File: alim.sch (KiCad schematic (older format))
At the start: 22 parts, among them IC10 74LS138, IC11 74LS138, IC12 74LS139, IC2 74LS09, IC5 74LS123, IC6 74LS393, IC7 74LS14, IC8 74LS04, IC9 74LS11

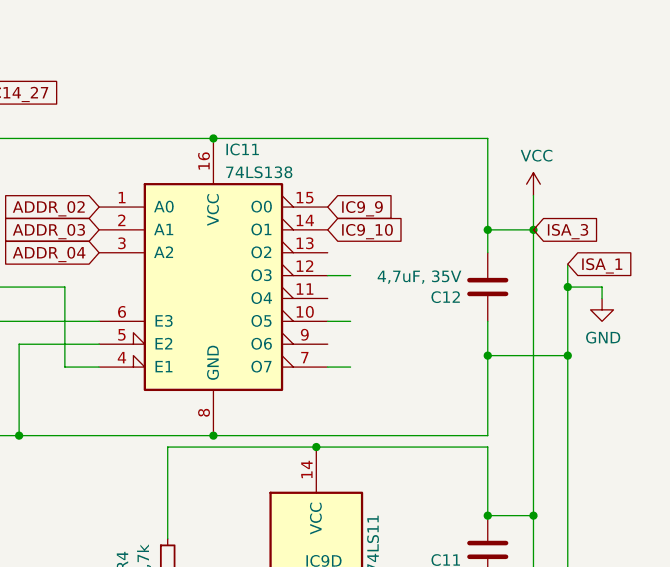
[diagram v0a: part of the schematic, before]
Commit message: les jumpers
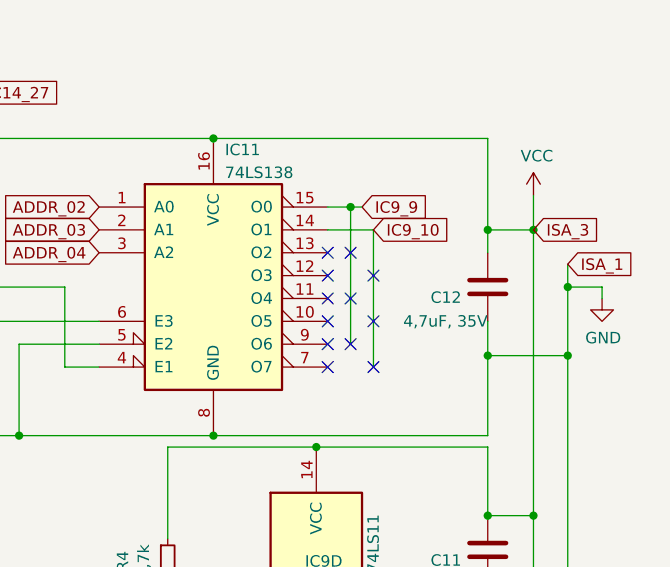
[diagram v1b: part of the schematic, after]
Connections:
- wire segments 122 -> 124
- no-connect marks 0 -> 12
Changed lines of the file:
@@
 AR Path="/61BDF4AD/6132D899" Ref="C12"  Part="1"
 F 0 "C12" H 6765 1896 50  0000 L CNN
-F 1 "4,7uF, 35V" H 6765 1805 50  0000 L CNN
+F 1 "4,7uF, 35V" H 6650 2000 50  0000 L CNN
 F 2 "Capacitor_THT:C_Disc_D4.3mm_W1.9mm_P5.00mm" H 6688 1700 50  0001 C CNN
 F 3 "~" H 6650 1850 50  0001 C CNN
@@
 Wire Wire Line
 	6650 1200 6650 1600
-Text GLabel 5950 1500 2    50   Input ~ 0
+Text GLabel 6100 1500 2    50   Input ~ 0
 IC9_9
 Connection ~ 5450 1200
@@
 Wire Wire Line
 	3550 1500 3800 1500
-Text GLabel 5950 1600 2    50   Input ~ 0
+Text GLabel 6150 1600 2    50   Input ~ 0
 IC9_10
 Wire Wire Line
@@
 Text GLabel 5500 4950 0    50   Input ~ 0
 DDD
-Wire Wire Line
-	5950 2000 6050 2000
-Wire Wire Line
-	5950 2200 6050 2200
-Wire Wire Line
-	5950 1800 6050 1800
+NoConn ~ 5950 2200
+NoConn ~ 5950 2000
+NoConn ~ 5950 1800
+NoConn ~ 6150 1800
+NoConn ~ 6150 2000
+NoConn ~ 6150 2200
+Wire Wire Line
+	6150 1600 6150 2200
+Wire Wire Line
+	5950 1600 6150 1600
+Wire Wire Line
+	6100 1500 6050 1500
+Wire Wire Line
+	6050 1500 6050 2100
+Connection ~ 6050 1500
+Wire Wire Line
+	6050 1500 5950 1500
+NoConn ~ 5950 1700
+NoConn ~ 6050 1700
+NoConn ~ 5950 1900
+NoConn ~ 6050 1900
+NoConn ~ 5950 2100
+NoConn ~ 6050 2100
 $EndSCHEMATC

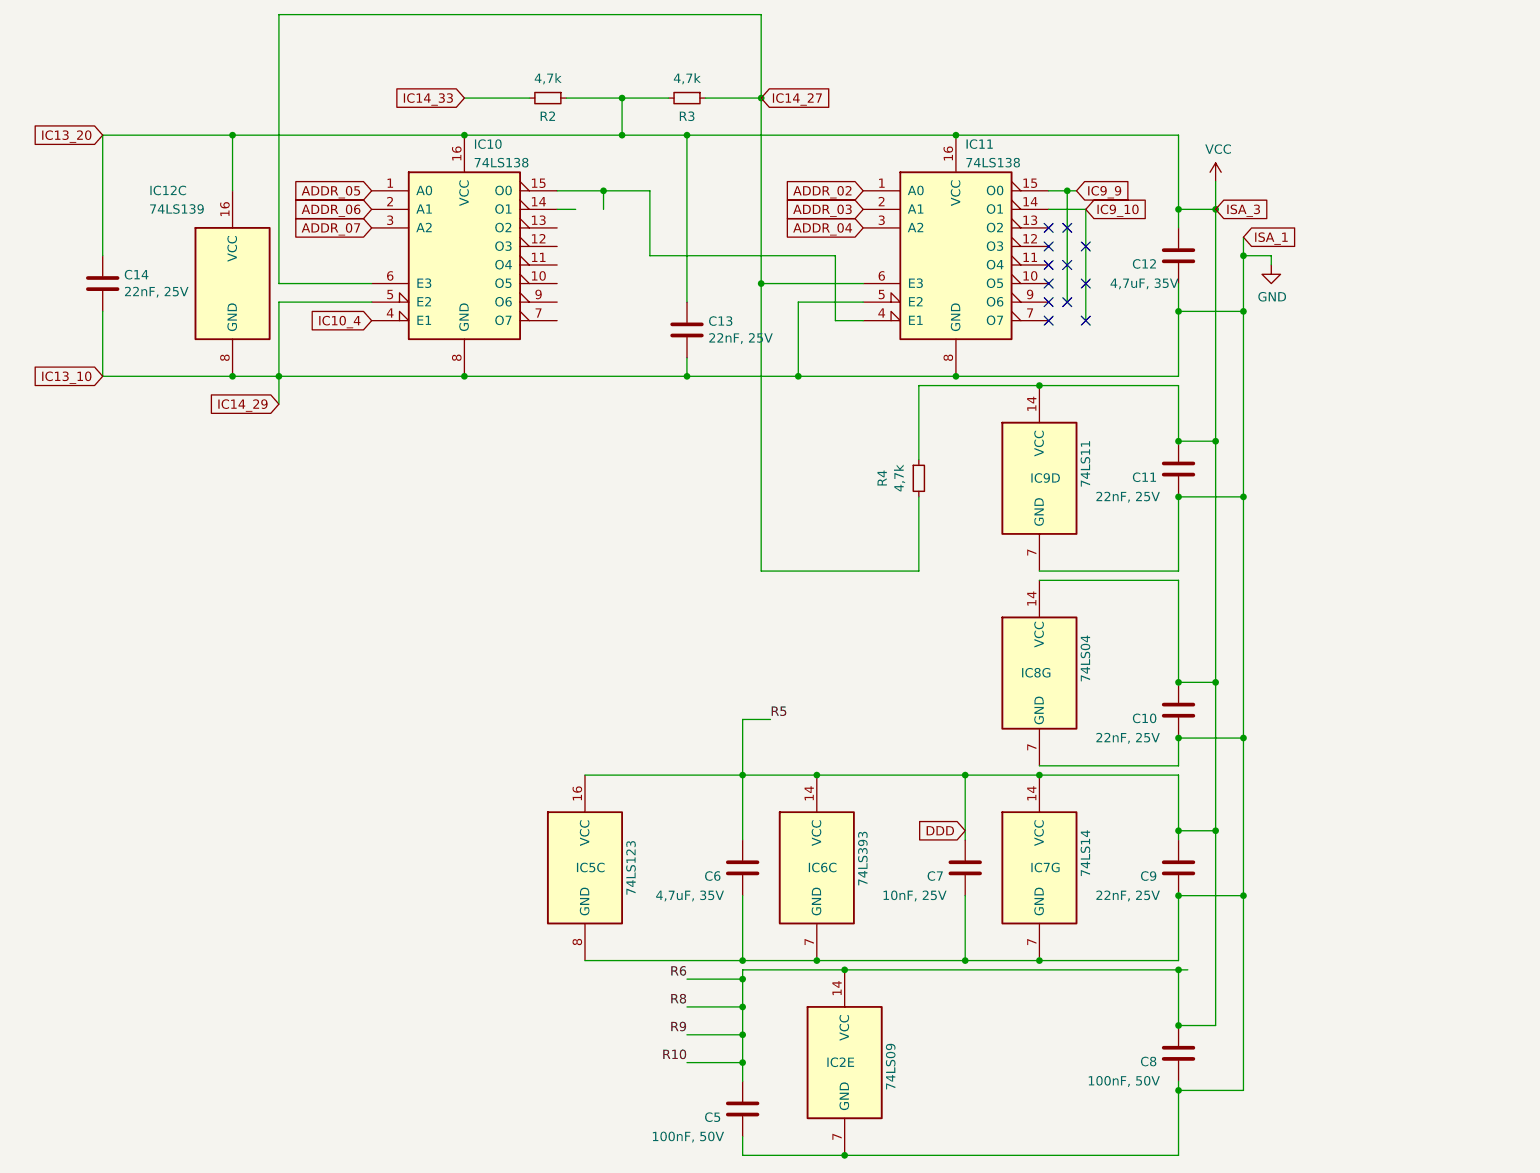
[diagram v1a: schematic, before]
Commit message: Schema de Freddy
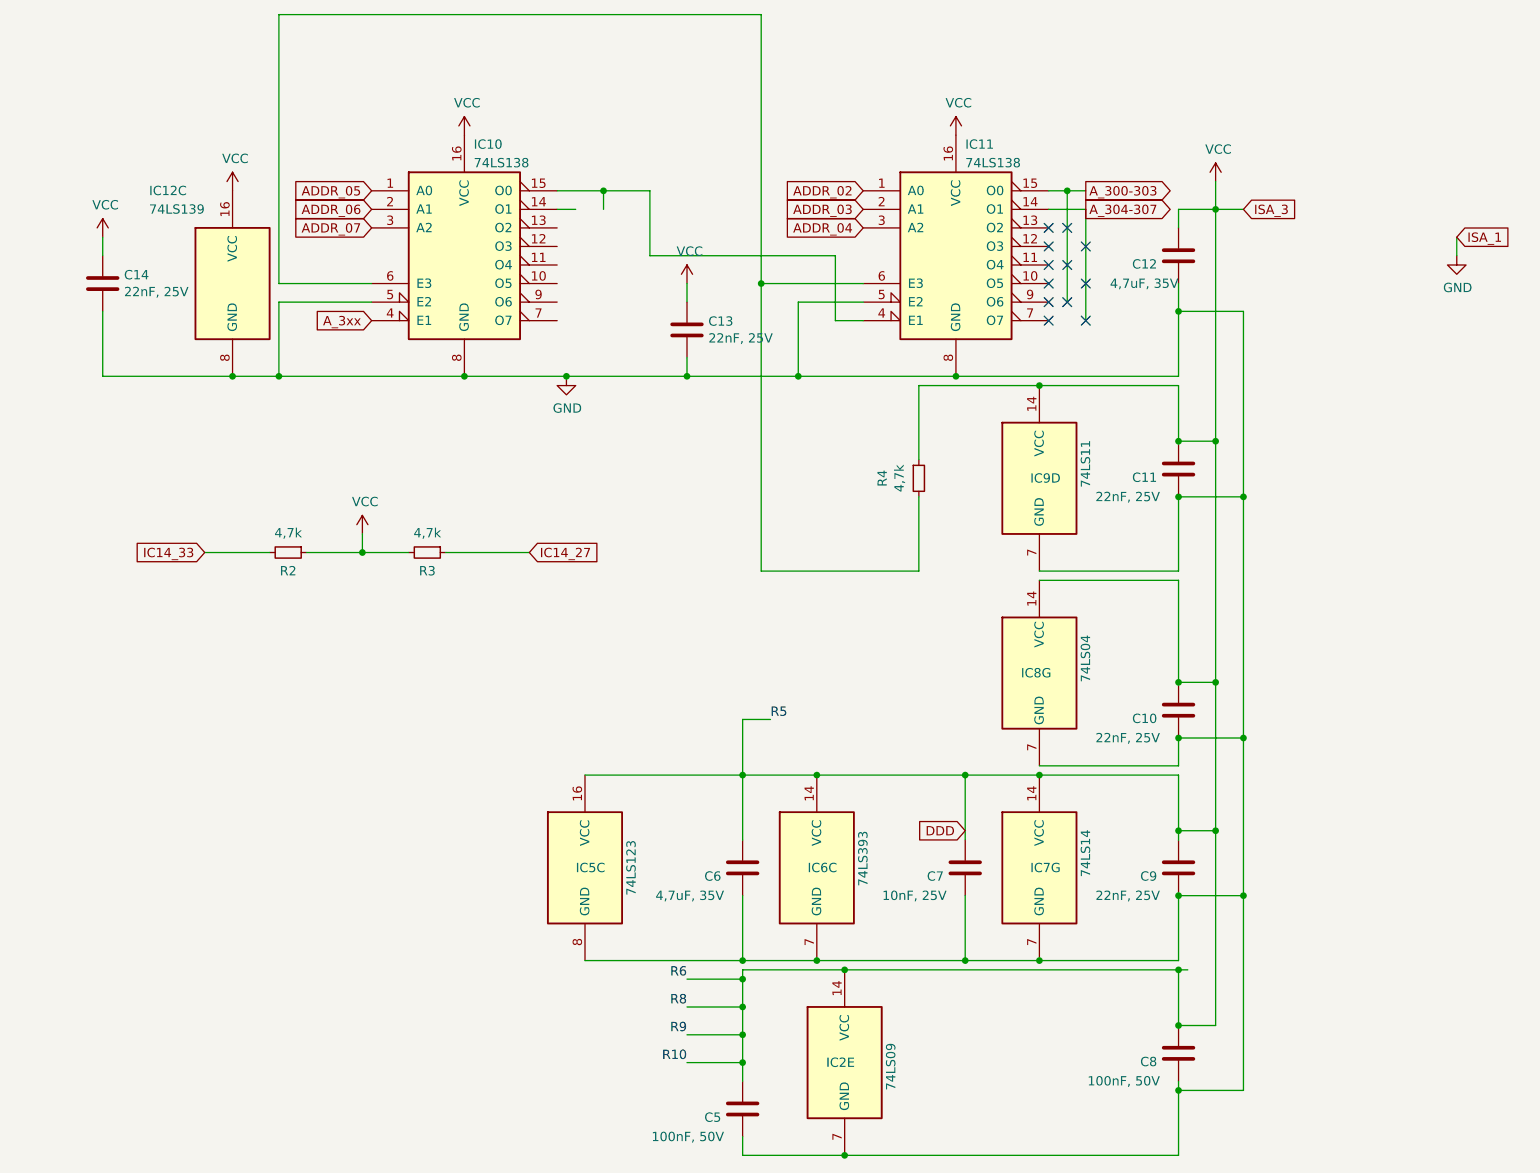
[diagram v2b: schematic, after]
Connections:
- net labels added: A_300-303, A_304-307, A_3xx
- net labels removed: IC10_4, IC13_10, IC13_20, IC14_29, IC9_10, IC9_9
- wire segments 124 -> 113
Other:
- moved on the sheet: R2, R3
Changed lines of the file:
@@
 $Descr A4 11693 8268
 encoding utf-8
-Sheet 3 3
+Sheet 1 1
 Title ""
 Date ""
@@
 L power:GND #PWR?
 U 1 1 612D8F44
-P 7150 1900
-F 0 "#PWR?" H 7150 1650 50  0001 C CNN
-F 1 "GND" H 7155 1727 50  0000 C CNN
-F 2 "" H 7150 1900 50  0001 C CNN
-F 3 "" H 7150 1900 50  0001 C CNN
-	1    7150 1900
+P 3350 2500
+F 0 "#PWR?" H 3350 2250 50  0001 C CNN
+F 1 "GND" H 3355 2327 50  0000 C CNN
+F 2 "" H 3350 2500 50  0001 C CNN
+F 3 "" H 3350 2500 50  0001 C CNN
+	1    3350 2500
 	1    0    0    -1
 $EndComp
@@
 	6650 2850 6850 2850
 Connection ~ 6650 2850
-Text GLabel 7000 1750 2    50   Input ~ 0
+Text GLabel 8150 1750 2    50   Input ~ 0
 ISA_1
-Text GLabel 6850 1600 2    50   Input ~ 0
+Text GLabel 7000 1600 2    50   Input ~ 0
 ISA_3
 $Comp
 L Device:R_Small R?
 U 1 1 6132D869
-P 4000 1000
+P 2600 3450
 AR Path="/6126F7E9/6132D869" Ref="R?"  Part="1"
 AR Path="/61BDF4AD/6132D869" Ref="R3"  Part="1"
-F 0 "R3" V 4100 1000 50  0000 C CNN
-F 1 "4,7k" V 3895 1000 50  0000 C CNN
-F 2 "Resistor_THT:R_Axial_DIN0309_L9.0mm_D3.2mm_P12.70mm_Horizontal" H 4000 1000 50  0001 C CNN
-F 3 "~" H 4000 1000 50  0001 C CNN
-	1    4000 1000
+F 0 "R3" V 2700 3450 50  0000 C CNN
+F 1 "4,7k" V 2495 3450 50  0000 C CNN
+F 2 "Resistor_THT:R_Axial_DIN0309_L9.0mm_D3.2mm_P12.70mm_Horizontal" H 2600 3450 50  0001 C CNN
+F 3 "~" H 2600 3450 50  0001 C CNN
+	1    2600 3450
 	0    1    1    0
 $EndComp
@@
 AR Path="/6126F7E9/6132D88D" Ref="IC?"  Part="1"
 AR Path="/61BDF4AD/6132D88D" Ref="IC11"  Part="1"
+AR Path="/6132D88D" Ref="IC11"  Part="1"
 F 0 "IC11" H 5500 2350 50  0000 L CNN
 F 1 "74LS138" H 5500 2250 50  0000 L CNN
@@
 $EndComp
 Wire Wire Line
-	1550 1500 1550 1200
-Wire Wire Line
 	1800 2000 2300 2000
 Wire Wire Line
@@
 	1800 2500 2800 2500
 Wire Wire Line
-	2800 1200 3650 1200
-Connection ~ 2800 1200
-Connection ~ 3650 1200
-Wire Wire Line
-	4000 1200 4000 2100
-Text GLabel 4400 1000 2    50   Input ~ 0
-IC14_27
+	4000 2000 4000 2100
 Wire Wire Line
 	4850 5700 6650 5700
@@
 Wire Wire Line
 	4850 6700 6650 6700
-Wire Wire Line
-	7150 1850 7000 1850
 Connection ~ 6850 4950
 Wire Wire Line
@@
 Wire Wire Line
 	6650 2000 6650 2150
-Wire Wire Line
-	7000 1850 7000 2150
 Connection ~ 7000 3150
 Connection ~ 6850 2850
 Wire Wire Line
 	6850 1450 6850 1600
-Wire Wire Line
-	6650 1200 6650 1600
-Text GLabel 6100 1500 2    50   Input ~ 0
-IC9_9
-Connection ~ 5450 1200
-Wire Wire Line
-	5450 1200 6650 1200
+Text GLabel 6150 1500 2    50   Output ~ 0
+A_300-303
 Connection ~ 5450 2500
 Wire Wire Line
 	5450 2500 6650 2500
-Wire Wire Line
-	3650 1200 4000 1200
 Wire Wire Line
 	4600 2100 4600 2500
@@
 	4600 2500 5450 2500
 Wire Wire Line
-	4400 2000 4400 1000
-Wire Wire Line
 	5900 2550 5250 2550
 Wire Wire Line
@@
 Wire Wire Line
 	4400 3550 5250 3550
-Connection ~ 4400 2000
-Wire Wire Line
-	4400 2000 4950 2000
 $Comp
 L Device:R_Small R?
 U 1 1 614CCF22
-P 3250 1000
+P 1850 3450
 AR Path="/6126F7E9/614CCF22" Ref="R?"  Part="1"
 AR Path="/61BDF4AD/614CCF22" Ref="R2"  Part="1"
-F 0 "R2" V 3350 1000 50  0000 C CNN
-F 1 "4,7k" V 3145 1000 50  0000 C CNN
-F 2 "Resistor_THT:R_Axial_DIN0309_L9.0mm_D3.2mm_P12.70mm_Horizontal" H 3250 1000 50  0001 C CNN
-F 3 "~" H 3250 1000 50  0001 C CNN
-	1    3250 1000
+F 0 "R2" V 1950 3450 50  0000 C CNN
+F 1 "4,7k" V 1745 3450 50  0000 C CNN
+F 2 "Resistor_THT:R_Axial_DIN0309_L9.0mm_D3.2mm_P12.70mm_Horizontal" H 1850 3450 50  0001 C CNN
+F 3 "~" H 1850 3450 50  0001 C CNN
+	1    1850 3450
 	0    1    1    0
 $EndComp
 Wire Wire Line
 	7000 2150 6650 2150
-Connection ~ 7000 2150
 Wire Wire Line
 	7000 2150 7000 3150
@@
 Wire Wire Line
 	6650 1600 6850 1600
-Connection ~ 6650 1600
 Wire Wire Line
 	6650 1600 6650 1700
@@
 	6850 1600 6850 2850
 Wire Wire Line
-	4100 1000 4400 1000
-Wire Wire Line
-	3900 1000 3650 1000
-Wire Wire Line
-	3650 1000 3650 1200
-Wire Wire Line
-	3650 1000 3350 1000
-Connection ~ 3650 1000
-Text GLabel 2800 1000 0    50   Input ~ 0
+	2500 3450 2250 3450
+Wire Wire Line
+	2250 3450 1950 3450
+Connection ~ 2250 3450
+Text GLabel 1400 3450 0    50   Input ~ 0
 IC14_33
 Wire Wire Line
-	3150 1000 2800 1000
-Wire Wire Line
-	850  1200 850  1850
+	1750 3450 1400 3450
+Wire Wire Line
+	850  1750 850  1850
 Text GLabel 2300 2200 0    50   Input ~ 0
-IC10_4
-Connection ~ 4000 1200
-Wire Wire Line
-	4000 1200 5450 1200
+A_3xx
 Connection ~ 4000 2500
 Wire Wire Line
 	4000 2500 4600 2500
 Wire Wire Line
-	2800 2500 4000 2500
+	2800 2500 3350 2500
 Wire Wire Line
 	3550 1500 3550 1600
@@
 Wire Wire Line
 	3550 1500 3800 1500
-Text GLabel 6150 1600 2    50   Input ~ 0
-IC9_10
+Text GLabel 6150 1600 2    50   Output ~ 0
+A_304-307
 Wire Wire Line
 	7000 6350 6650 6350
@@
 Wire Wire Line
 	850  2500 1550 2500
-Connection ~ 1550 1200
-Wire Wire Line
-	1550 1200 2800 1200
-Wire Wire Line
-	850  1200 1550 1200
-Wire Wire Line
-	1800 2500 1800 2650
-Text GLabel 1800 2650 0    50   Input ~ 0
-IC14_29
-Text GLabel 850  2500 0    50   Input ~ 0
-IC13_10
-Text GLabel 850  1200 0    50   Input ~ 0
-IC13_20
 Wire Wire Line
 	1800 550  4400 550
 Wire Wire Line
-	4400 550  4400 1000
-Wire Wire Line
 	1800 550  1800 2000
-Connection ~ 4400 1000
-Wire Wire Line
-	7000 1750 7000 1850
-Connection ~ 7000 1850
-Wire Wire Line
-	7150 1850 7150 1900
+Wire Wire Line
+	8150 1750 8150 1850
 Text GLabel 5500 4950 0    50   Input ~ 0
 DDD
@@
 	5950 1600 6150 1600
 Wire Wire Line
-	6100 1500 6050 1500
+	6150 1500 6050 1500
 Wire Wire Line
 	6050 1500 6050 2100
@@
 NoConn ~ 5950 2100
 NoConn ~ 6050 2100
+Connection ~ 3350 2500
+Wire Wire Line
+	3350 2500 4000 2500
+$Comp
+L power:GND #PWR?
+U 1 1 61332220
+P 8150 1850
+F 0 "#PWR?" H 8150 1600 50  0001 C CNN
+F 1 "GND" H 8155 1677 50  0000 C CNN
+F 2 "" H 8150 1850 50  0001 C CNN
+F 3 "" H 8150 1850 50  0001 C CNN
+	1    8150 1850
+	1    0    0    -1
+$EndComp
+Wire Wire Line
+	7000 1600 6850 1600
+$Comp
+L power:VCC #PWR?
+U 1 1 6134655A
+P 5450 1200
+F 0 "#PWR?" H 5450 1050 50  0001 C CNN
+F 1 "VCC" H 5465 1373 50  0000 C CNN
+F 2 "" H 5450 1200 50  0001 C CNN
+F 3 "" H 5450 1200 50  0001 C CNN
+	1    5450 1200
+	1    0    0    -1
+$EndComp
+$Comp
+L power:VCC #PWR?
+U 1 1 6134C22C
+P 2250 3350
+F 0 "#PWR?" H 2250 3200 50  0001 C CNN
+F 1 "VCC" H 2265 3523 50  0000 C CNN
+F 2 "" H 2250 3350 50  0001 C CNN
+F 3 "" H 2250 3350 50  0001 C CNN
+	1    2250 3350
+	1    0    0    -1
+$EndComp
+Wire Wire Line
+	2250 3350 2250 3450
+$Comp
+L power:VCC #PWR?
+U 1 1 61355045
+P 4000 2000
+F 0 "#PWR?" H 4000 1850 50  0001 C CNN
+F 1 "VCC" H 4015 2173 50  0000 C CNN
+F 2 "" H 4000 2000 50  0001 C CNN
+F 3 "" H 4000 2000 50  0001 C CNN
+	1    4000 2000
+	1    0    0    -1
+$EndComp
+$Comp
+L power:VCC #PWR?
+U 1 1 61356035
+P 2800 1200
+F 0 "#PWR?" H 2800 1050 50  0001 C CNN
+F 1 "VCC" H 2815 1373 50  0000 C CNN
+F 2 "" H 2800 1200 50  0001 C CNN
+F 3 "" H 2800 1200 50  0001 C CNN
+	1    2800 1200
+	1    0    0    -1
+$EndComp
+Text GLabel 3150 3450 2    50   Input ~ 0
+IC14_27
+Wire Wire Line
+	3150 3450 2700 3450
+Wire Wire Line
+	4400 550  4400 2000
+Connection ~ 4400 2000
+Wire Wire Line
+	4400 2000 4950 2000
+$Comp
+L power:VCC #PWR?
+U 1 1 6137A5D8
+P 1550 1500
+F 0 "#PWR?" H 1550 1350 50  0001 C CNN
+F 1 "VCC" H 1565 1673 50  0000 C CNN
+F 2 "" H 1550 1500 50  0001 C CNN
+F 3 "" H 1550 1500 50  0001 C CNN
+	1    1550 1500
+	1    0    0    -1
+$EndComp
+$Comp
+L power:VCC #PWR?
+U 1 1 6137B0FA
+P 850 1750
+F 0 "#PWR?" H 850 1600 50  0001 C CNN
+F 1 "VCC" H 865 1923 50  0000 C CNN
+F 2 "" H 850 1750 50  0001 C CNN
+F 3 "" H 850 1750 50  0001 C CNN
+	1    850  1750
+	1    0    0    -1
+$EndComp
 $EndSCHEMATC

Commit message: Dernière version de Freddy
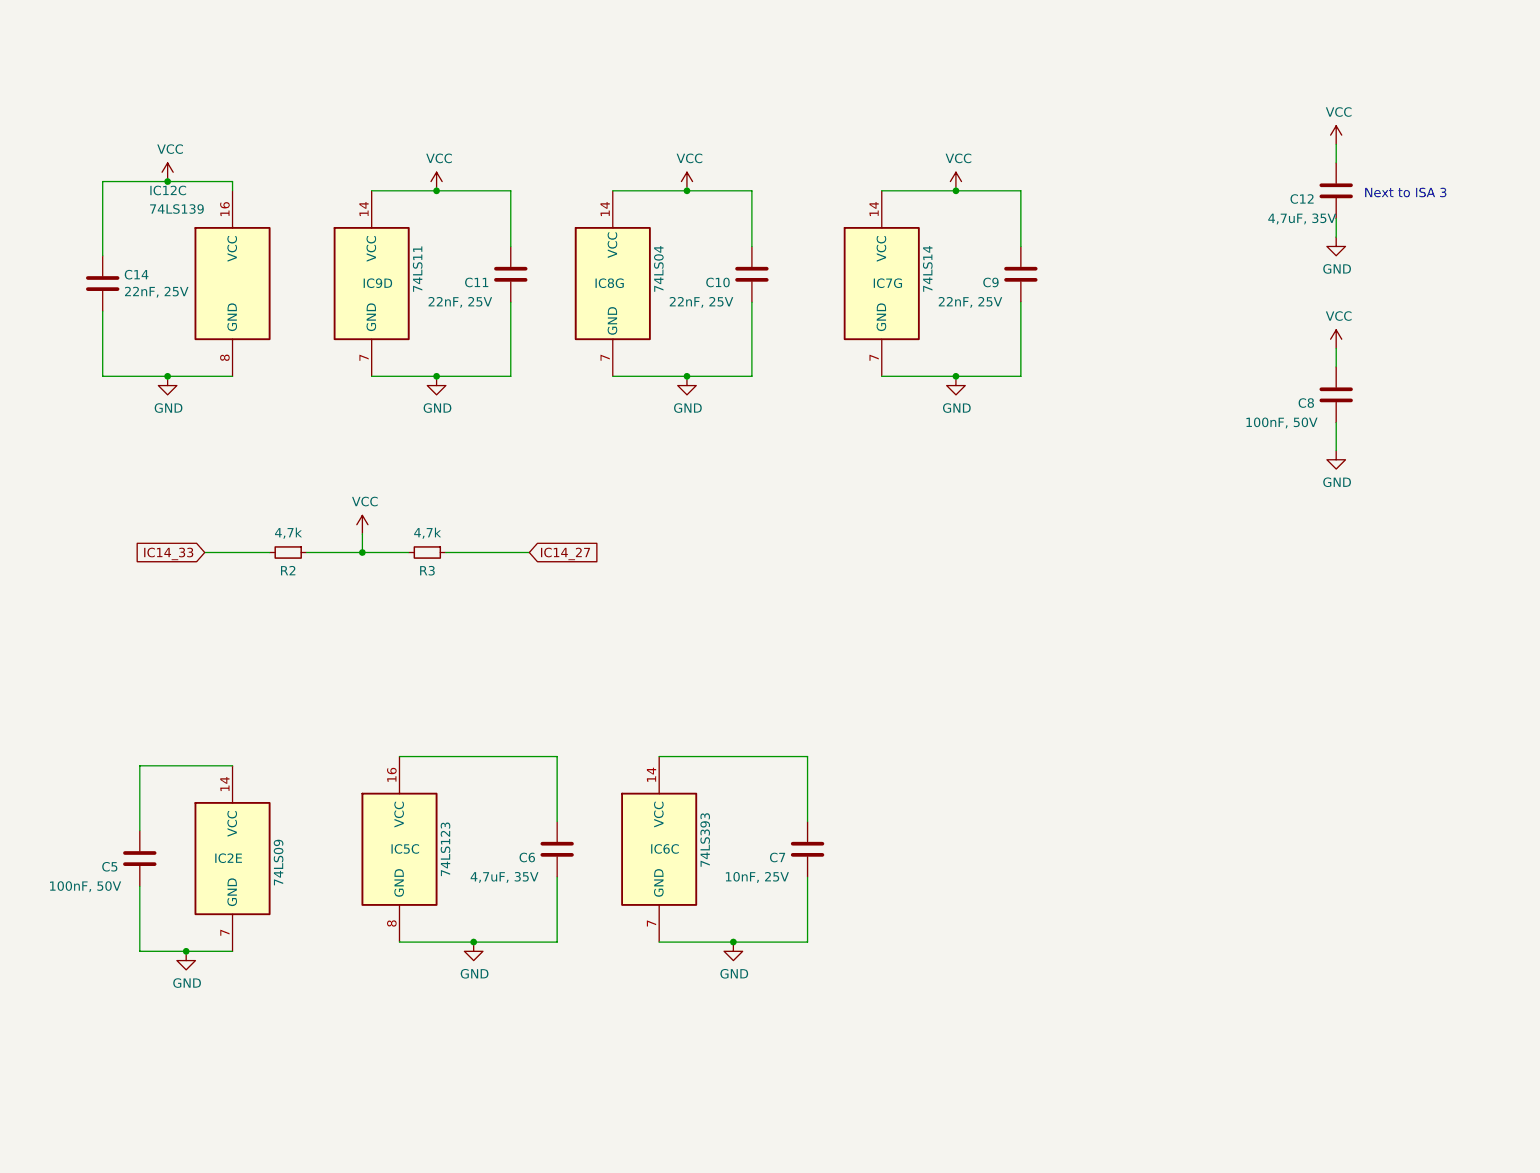
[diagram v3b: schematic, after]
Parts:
- removed C13: 22nF, 25V, Capacitor_THT:C_Disc_D4.3mm_W1.9mm_P5.00mm, symbol Device:C
- removed IC10, IC11: 74LS138, Package_DIP:DIP-16_W7.62mm, symbol 74xx:74LS138
- removed R4: 4,7k, Resistor_THT:R_Axial_DIN0309_L9.0mm_D3.2mm_P12.70mm_Horizontal, symbol Device:R_Small
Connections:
- net labels removed: ADDR_02, ADDR_03, ADDR_04, ADDR_05, ADDR_06, ADDR_07, A_300-303, A_304-307, A_3xx, DDD, ISA_1, ISA_3, R10, R5, R6, R8, R9
- wire segments 113 -> 49
- no-connect marks 12 -> 0
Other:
- note added: "Next to ISA 3"
- moved on the sheet: C10, C11, C12, C5, C6, C7, C8, C9, IC2E, IC5C, IC6C, IC7G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
